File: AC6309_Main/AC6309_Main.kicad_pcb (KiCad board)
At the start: 2 copper layers, 99.1 x 99.1 mm, 23 parts, among them J3 FTDI Header, J4 Conn_IO, SW1 Reset, U1 HD63B09P, U2 W24257, U3 28C256, U4 HD63B50, U5 74HCT00, U6 74HC138, Y1 7.3728 MHz

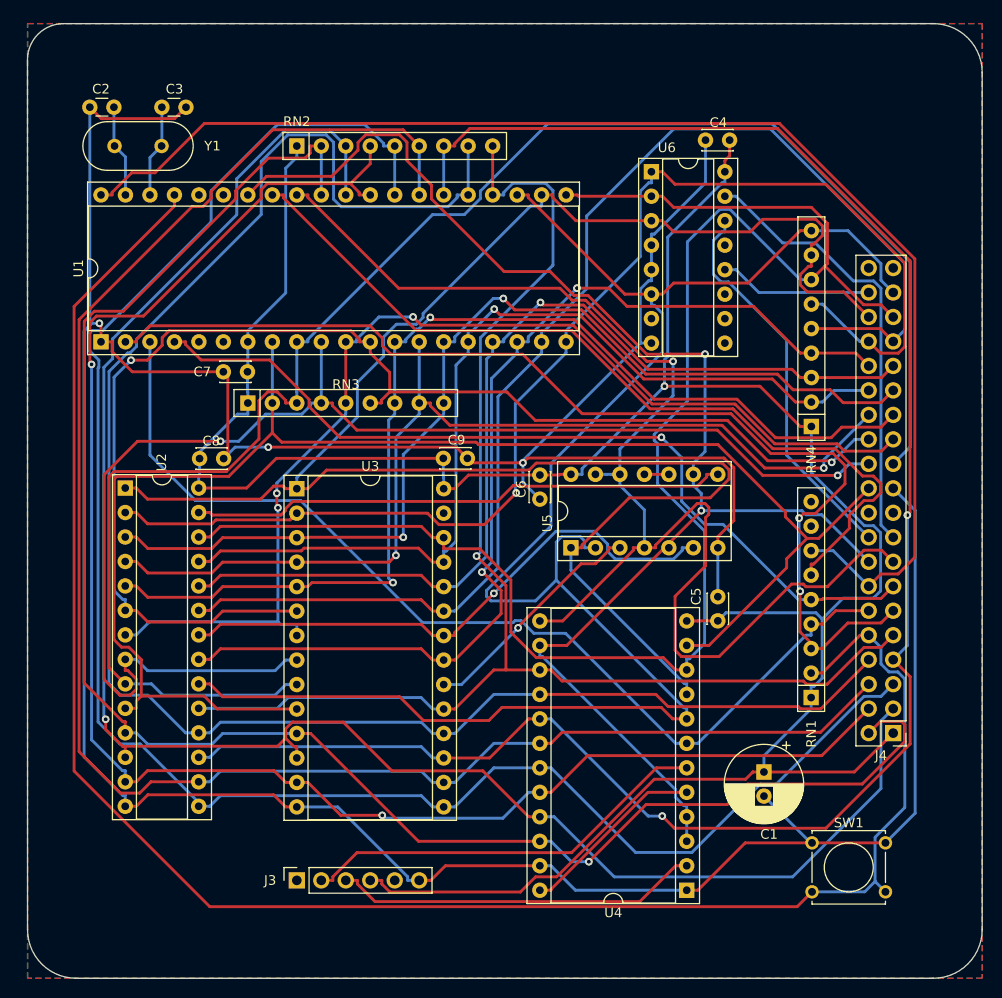
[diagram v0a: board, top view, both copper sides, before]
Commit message: Updates from 2024. Rev1 going in production.
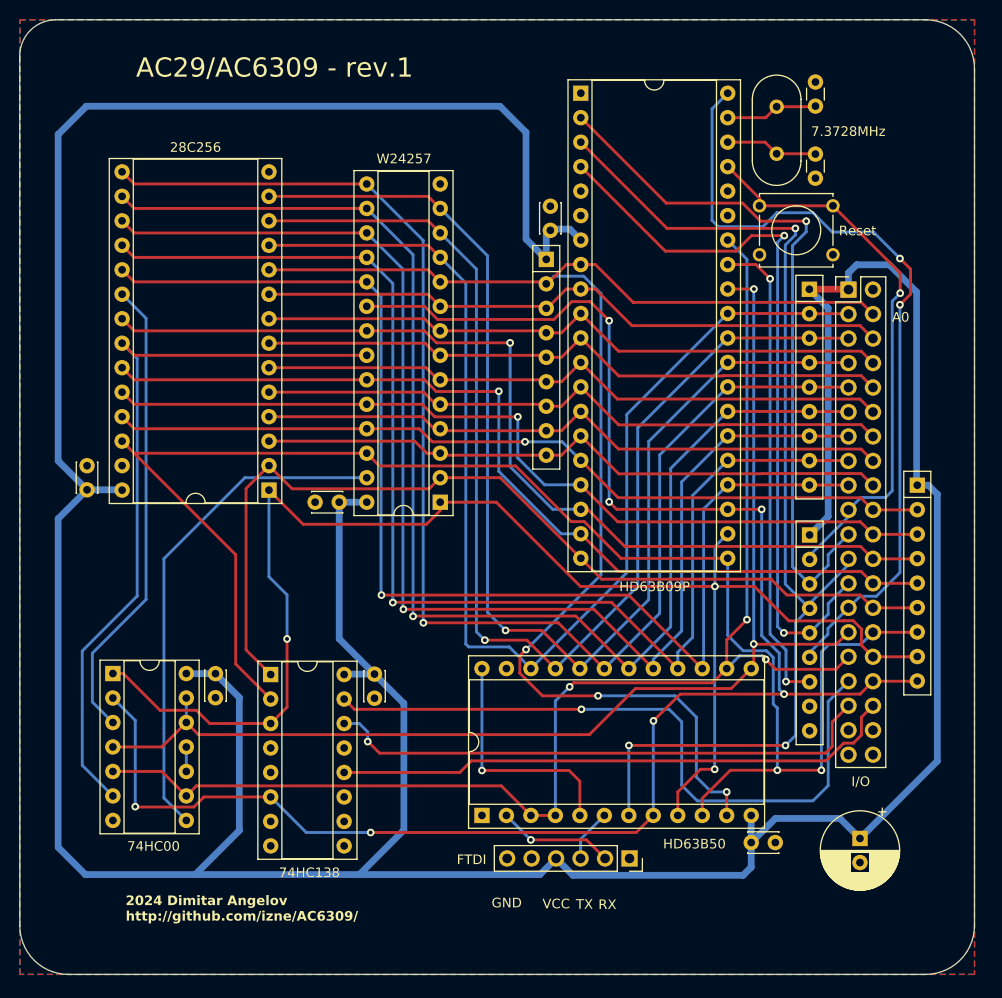
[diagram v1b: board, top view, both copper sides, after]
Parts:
- J1: renamed from J4; value Conn_IO -> I/O
- J2: renamed from J3; value FTDI Header -> FTDI
- U5: value 74HCT00 -> 74HC00
- moved C2 72.8 mm to (132.6, 34.0), turned to 90 degrees
- moved C3 68.0 mm to (132.6, 38.9), turned to -90 degrees
- moved C4 66.5 mm to (86.8, 92.9), turned to -90 degrees
- moved U6 65.4 mm to (76.0, 92.9)
- moved Y1 63.8 mm to (128.5, 38.9), turned to 90 degrees
- moved SW1 61.1 mm to (134.4, 49.4), turned to 180 degrees
- moved U1 56.1 mm to (108.2, 32.6), turned to 0 degrees
- moved RN2 55.2 mm to (131.9, 53.0), turned to -90 degrees
- moved U5 49.3 mm to (59.7, 92.8), turned to 0 degrees
- moved J1 46.3 mm to (136.0, 53.0), turned to 0 degrees
- moved C6 39.5 mm to (70.3, 92.8)
- moved C9 37.1 mm to (57.0, 73.8), turned to 90 degrees
- moved C7 34.7 mm to (105.0, 46.9), turned to 90 degrees
- moved J2 34.6 mm to (113.3, 112.0), turned to -90 degrees
- moved RN3 34.4 mm to (104.6, 49.9), turned to -90 degrees
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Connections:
- J1 pad 10: //RESET -> /A3
- J1 pad 11: //NMI -> /D4
- J1 pad 12: //IRQ -> /A4
- J1 pad 13: //FIRQ -> /D5
- J1 pad 14: //HALT -> /A5
- J1 pad 15: /R/W -> /D6
- J1 pad 16: /E -> /A6
- J1 pad 17: //8000_CS -> /D7
- J1 pad 18: //9000_CS -> /A7
- J1 pad 19: unconnected-(J4-Pin_19-Pad19) -> //RESET
- J1 pad 2: /D0 -> GND
- J1 pad 20: unconnected-(J4-Pin_20-Pad20) -> /A8
- J1 pad 21: GND -> //NMI
- J1 pad 22: /A0 -> /A9
- J1 pad 23: /A1 -> //IRQ
- J1 pad 24: /A2 -> /A10
- J1 pad 25: /A3 -> //FIRQ
- J1 pad 26: /A4 -> /A11
- J1 pad 27: /A5 -> //HALT
- J1 pad 28: /A6 -> /A12
- J1 pad 29: /A7 -> /R/W
- J1 pad 3: /D1 -> /D0
- J1 pad 30: /A8 -> /A13
- J1 pad 31: /A9 -> /E
- J1 pad 32: /A10 -> /A14
- J1 pad 33: /A11 -> //8000_CS
- J1 pad 34: /A12 -> /A15
- J1 pad 35: /A13 -> //9000_CS
- J1 pad 36: /A14 -> //B000_CS
- J1 pad 37: /A15 -> unconnected-(J1-Pin_37-Pad37)
- J1 pad 38: //B000_CS -> unconnected-(J1-Pin_38-Pad38)
- J1 pad 4: /D2 -> /A0
- J1 pad 5: /D3 -> /D1
- J1 pad 6: /D4 -> /A1
- J1 pad 7: /D5 -> /D2
- J1 pad 8: /D6 -> /A2
- J1 pad 9: /D7 -> /D3
- J2 pad 2: /ACIA_TX -> /ACIA_RX
- J2 pad 3: /ACIA_RX -> /ACIA_TX
- RN1 pad 6: //DMABREQ -> //HALT
- RN1 pad 7: //HALT -> //DMABREQ
- U1 pad 35: /Q -> unconnected-(U1-Q-Pad35)
- U6 pad 11: //C000_CS_ROM -> unconnected-(U6-~{Y4}-Pad11)
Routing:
- net GND: track 361.7 -> 0.00 mm, vias 3 -> 0
- net VCC: track 266.2 -> 424.8 mm, vias 1 -> 0
- net //RESET: track 192.2 -> 58.0 mm, vias 0 -> 1
- net /A1: track 174.6 -> 66.2 mm
- net /A2: track 140.9 -> 66.2 mm, vias 2 -> 0
- net /A4: track 135.7 -> 66.2 mm, vias 2 -> 0
- net /D1: track 188.0 -> 125.4 mm
- net /D5: track 196.4 -> 135.0 mm, vias 2 -> 1
- net /D0: track 181.4 -> 125.3 mm, vias 1 -> 0
- net //HALT: track 138.0 -> 83.4 mm, vias 0 -> 2
- net /D6: track 182.2 -> 131.6 mm, vias 0 -> 1
- net /D2: track 174.7 -> 124.9 mm, vias 2 -> 1
- net /A3: track 116.0 -> 66.3 mm, vias 3 -> 0
- net /D3: track 189.5 -> 141.7 mm, vias 0 -> 1
- net /A5: track 113.4 -> 66.3 mm, vias 2 -> 0
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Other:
- board text added: "2024 Dimitar Angelov http://github.com/izne/AC6309/"
- board text added: "7.3728MHz"
- board text added: "A0"
- board text added: "AC29/AC6309 - rev.1"
- board text added: "GND"
- board text added: "RX"
- board text added: "TX"
- board text added: "VCC"
